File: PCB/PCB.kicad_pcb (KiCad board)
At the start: 2 copper layers, 3 parts, among them U3 PC817, U4 MAX31855KASA

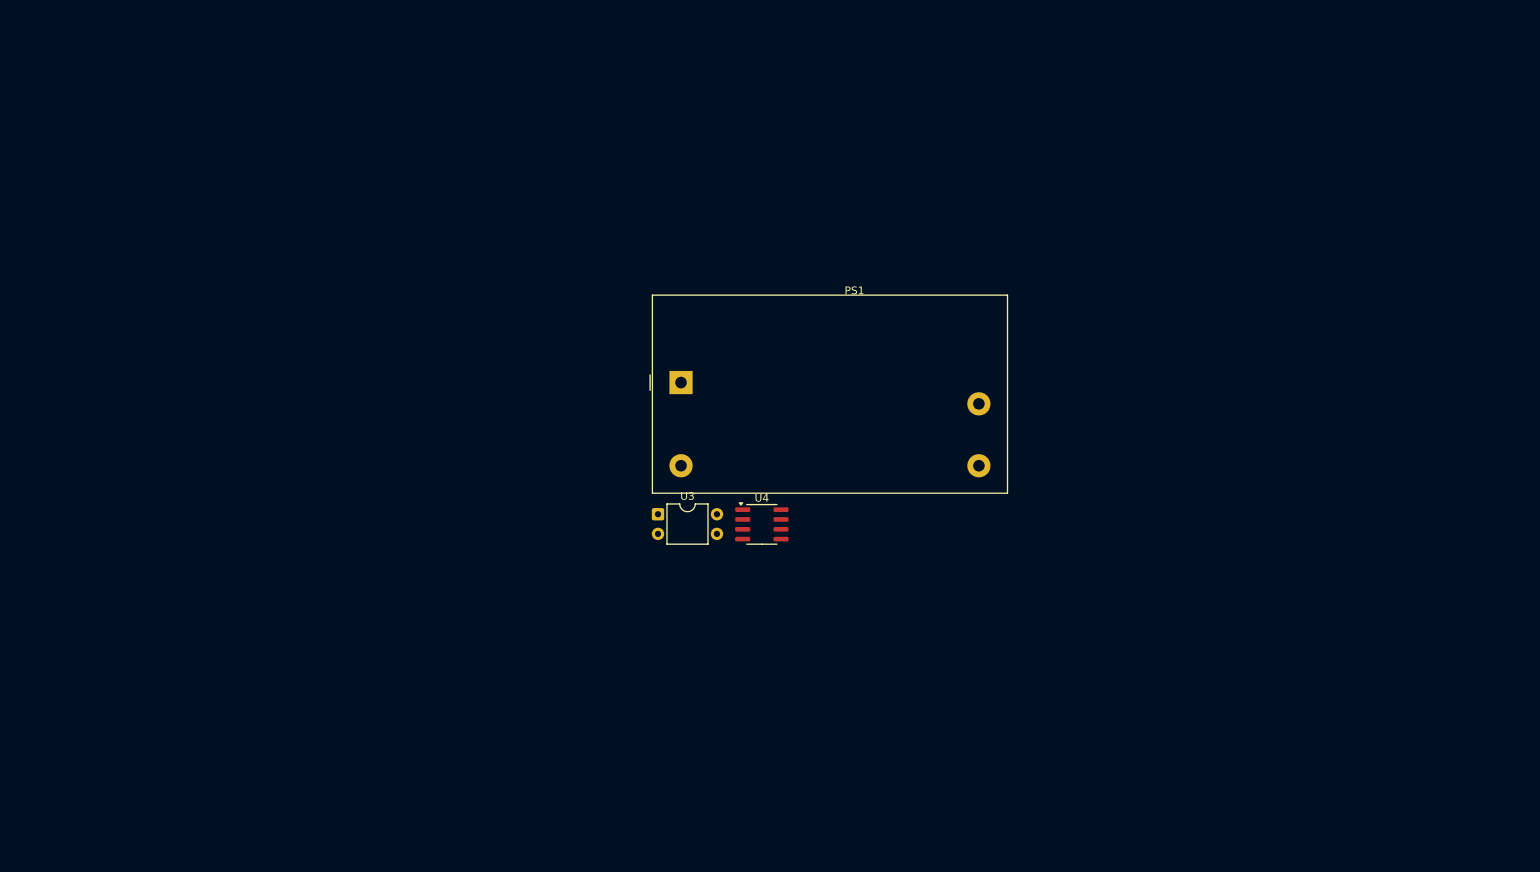
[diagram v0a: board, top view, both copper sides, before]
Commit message: add all the changes i've made, sorry for not gitting it bit by bit
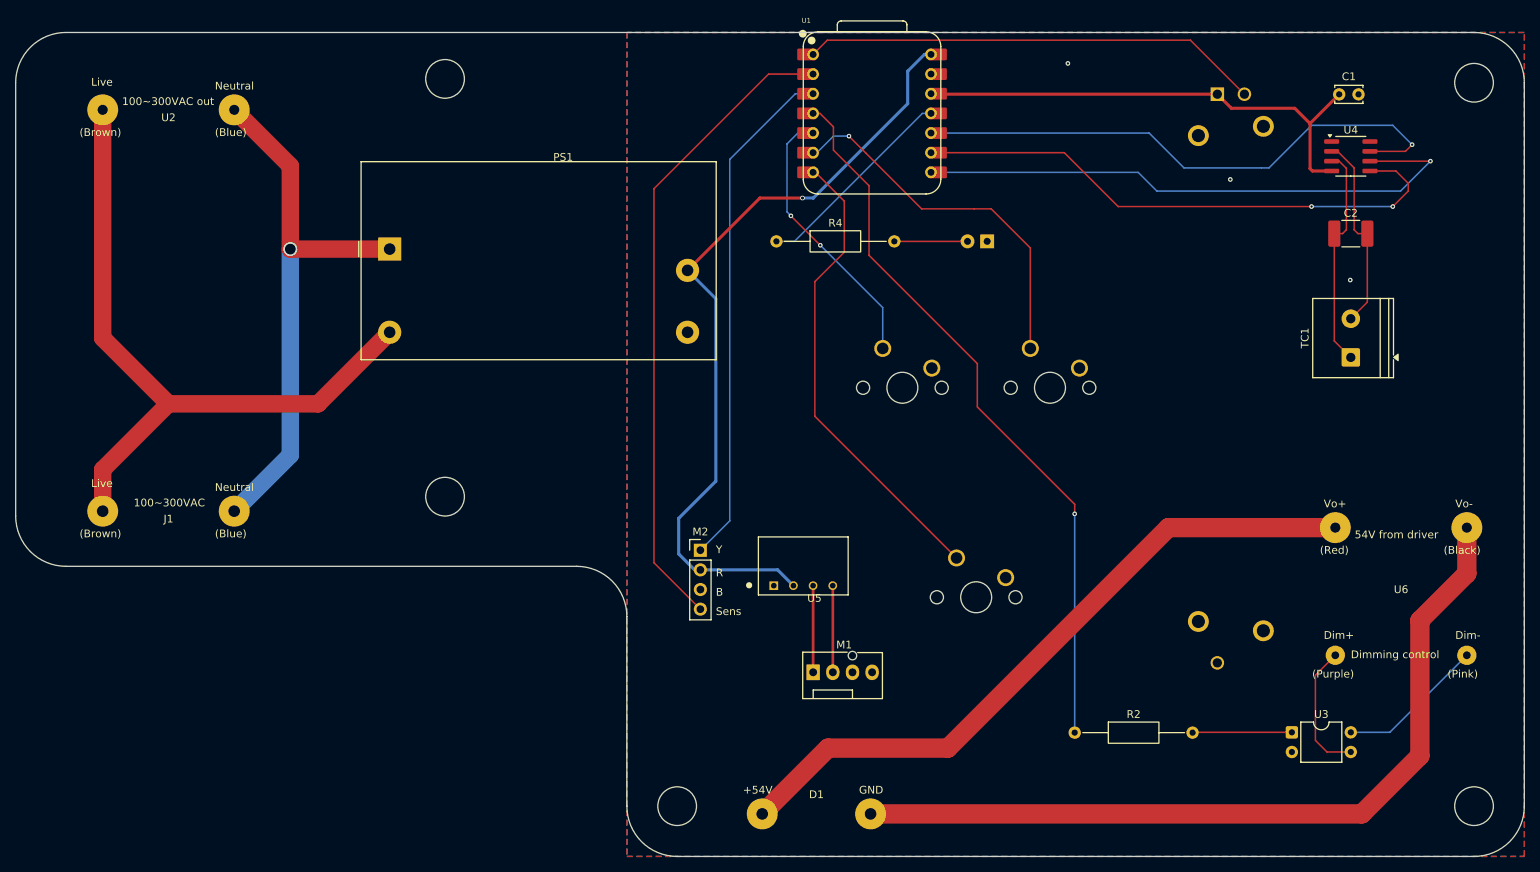
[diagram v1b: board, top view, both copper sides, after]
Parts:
- added C1: 0.1µF, Capacitor_THT:C_Disc_D3.4mm_W2.1mm_P2.50mm, F.Cu at (198.6, 40.0)
- added C2: 10nF, Capacitor_SMD:C_1812_4532Metric_Pad1.57x3.40mm_HandSolder, F.Cu at (200.1, 58.0)
- added D1: LED, custom footprints and stuff:Big Lumileds LED, F.Cu at (131.0, 137.5)
- added D2: LED red, LED_THT:LED_D5.0mm, B.Cu at (153.1, 59.0)
- added J1: IEC_C14_Receptacle, custom footprints and stuff:C14 Power input, F.Cu at (47.2, 97.9)
- added M1: Fan_4pin, Connector:FanPinHeader_1x04_P2.54mm_Vertical, F.Cu at (130.6, 114.7)
- added M2: Motor_Servo, Connector_PinHeader_2.54mm:PinHeader_1x04_P2.54mm_Vertical, F.Cu at (116.0, 98.9)
- added R2: 42Ω 0.12W, Resistor_THT:R_Axial_DIN0207_L6.3mm_D2.5mm_P15.24mm_Horizontal, F.Cu at (164.4, 122.5)
- added R4: 40-60Ω, Resistor_THT:R_Axial_DIN0207_L6.3mm_D2.5mm_P15.24mm_Horizontal, F.Cu at (125.8, 59.0)
- added RV1: Pot, Potentiometer_THT:Potentiometer_Bourns_PTA6043_Single_Slide, B.Cu at (182.8, 40.0)
- added SW2: SW_Push SET, Button_Switch_Keyboard:SW_Cherry_MX_1.00u_PCB, B.Cu at (149.1, 99.9)
- added SW3: SW_Push Pos1, Button_Switch_Keyboard:SW_Cherry_MX_1.00u_PCB, B.Cu at (158.7, 72.8)
- added SW4: SW_Push Pos2, Button_Switch_Keyboard:SW_Cherry_MX_1.00u_PCB, B.Cu at (139.6, 72.8)
- added TC1: Thermocouple_Block, TerminalBlock_Philmore:TerminalBlock_Philmore_TB132_1x02_P5.00mm_Horizontal, F.Cu at (200.1, 74.0)
- added U1: XIAO-RP2040-DIP, Seeed Studio XIAO Series Library:XIAO-RP2040-DIP, F.Cu at (138.2, 42.5)
- added U2: Meanwell ELG-150-54B AC Side, custom footprints and stuff:Meanwell ELG-150-54B AC side, F.Cu at (47.2, 46.0)
- added U5: SMU02L-12, SMU02L_12:SIP750W50P254L1160H1014Q4, F.Cu at (129.3, 101.0)
- added U6: Meanwell ELG-150-54B Other side, custom footprints and stuff:Meanwell ELG-150-54B Other Side, F.Cu at (206.6, 100.0)
- moved U4 89.8 mm to (200.1, 48.0)
- moved U3 86.6 mm to (192.4, 122.5)
- moved PS1 41.4 mm to (75.8, 60.0)
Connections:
- U4 pad 2: GND -> Net-(TC1--)
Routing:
- net Net-(D1-K): track 0.00 -> 106.1 mm
- net +5V: track 0.00 -> 102.2 mm, vias 0 -> 1
- net Net-(U1-GPIO29/ADC3/A3): track 0.00 -> 94.6 mm, vias 0 -> 1
- net Net-(J1-L): track 0.00 -> 91.3 mm
- net Net-(D1-A): track 0.00 -> 89.4 mm
- net Net-(M2-Sense): track 0.00 -> 82.7 mm
- net Net-(U1-GPIO1/RX): track 0.00 -> 75.0 mm, vias 0 -> 1
- net Net-(U1-GPIO4/MISO): track 0.00 -> 73.2 mm, vias 0 -> 1
- net Net-(U1-GPIO2/SCK): track 0.00 -> 71.2 mm, vias 0 -> 2
- net Net-(J1-N): track 0.00 -> 70.7 mm, vias 0 -> 1
- net Net-(M2-PWM): track 0.00 -> 66.4 mm
- net +3V3: track 0.00 -> 63.8 mm
- net Net-(U1-GPIO0/TX): track 0.00 -> 60.8 mm
- net Net-(U1-GPIO26/ADC0/A0): track 0.00 -> 59.4 mm
- net Net-(U1-GPIO7/SCL): track 0.00 -> 47.9 mm, vias 0 -> 1
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- added copper zone on B.Cu, net GND
- added copper zone on F.Cu, net GND
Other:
- board outline added: 195 x 106.5 mm

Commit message: uhh did stuff by the looks of it
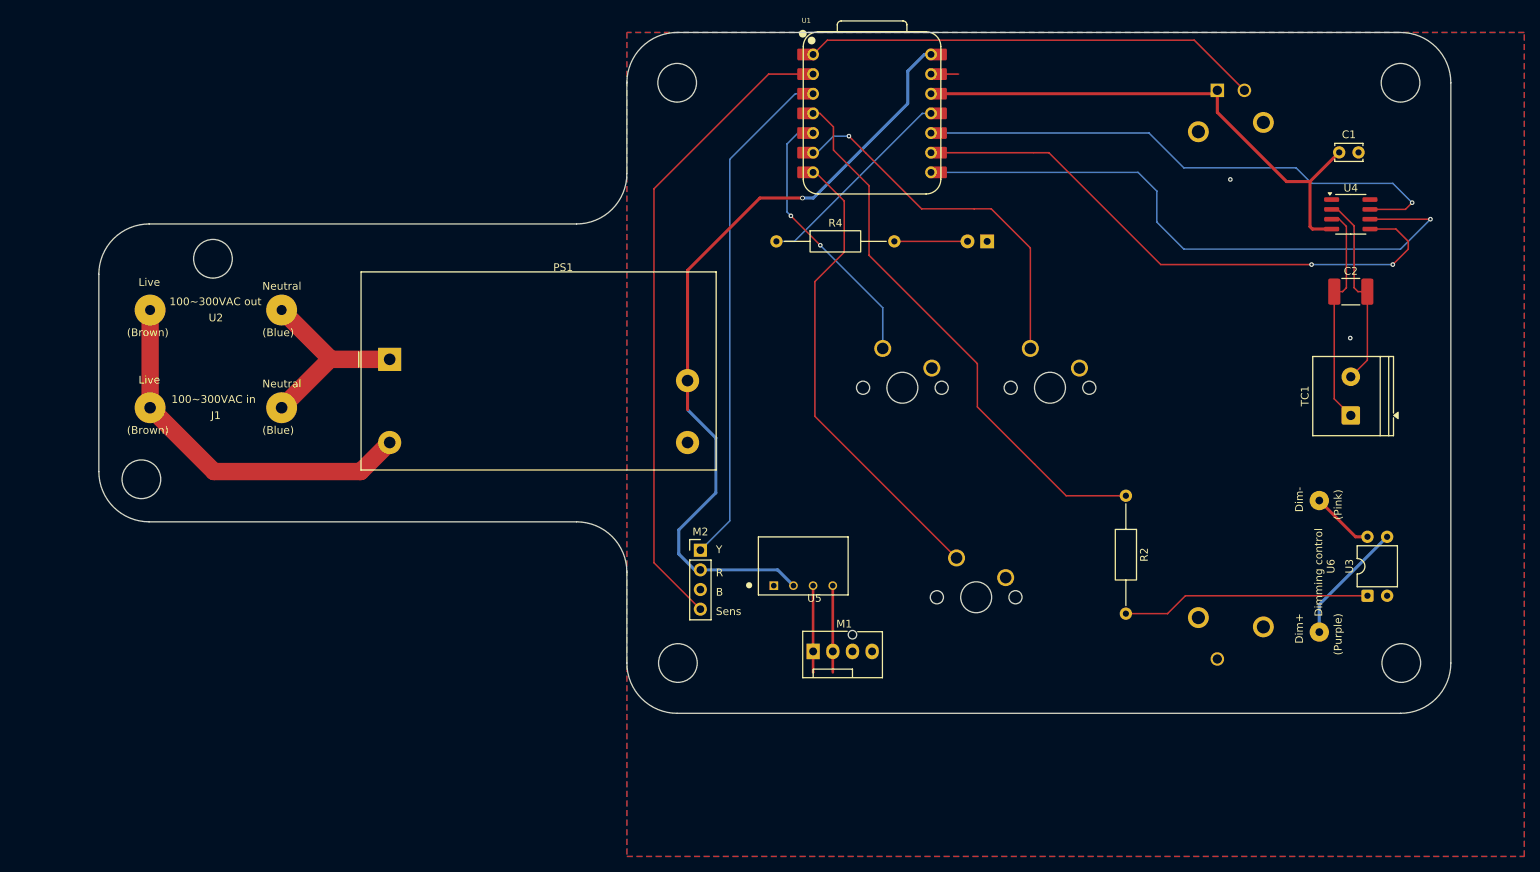
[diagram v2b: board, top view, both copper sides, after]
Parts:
- removed D1: LED, custom footprints and stuff:Big Lumileds LED
- moved R2 31.3 mm to (171.0, 91.9), turned to -90 degrees
- moved U2 26.6 mm to (53.4, 71.9)
- moved U6 23.1 mm to (183.5, 101.0), turned to 90 degrees
- moved U3 20.2 mm to (202.2, 104.8), turned to 90 degrees
- moved J1 14.7 mm to (53.4, 84.5)
- moved PS1 14.2 mm to (75.8, 74.2)
- moved C1 7.50 mm to (198.6, 47.5)
- moved C2 7.50 mm to (200.1, 65.5)
- moved TC1 7.50 mm to (200.1, 81.5)
- moved U4 7.50 mm to (200.1, 55.5)
- moved M1 2.70 mm to (130.6, 112.0)
- moved RV1 0.50 mm to (182.8, 39.5)
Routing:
- net Net-(D1-K): track 106.1 -> 0.00 mm
- net Net-(D1-A): track 89.4 -> 0.00 mm
- net Net-(J1-N): track 70.7 -> 25.6 mm, vias 1 -> 0
- net Net-(J1-L): track 91.3 -> 48.4 mm
- net Net-(U1-GPIO29/ADC3/A3): track 94.6 -> 71.2 mm, vias 1 -> 0
- net Net-(R2-Pad2): track 12.8 -> 32.2 mm
- net Net-(U6-Dim-): track 19.1 -> 8.17 mm
- net Net-(U1-GPIO1/RX): track 75.0 -> 80.4 mm
- net +3V3: track 63.8 -> 69.0 mm
- net Net-(U1-GPIO2/SCK): track 71.2 -> 74.3 mm
- net GND: track 0.00 -> 2.73 mm, vias 3 -> 2
- net Net-(U1-GPIO4/MISO): track 73.2 -> 71.7 mm
- net Net-(U6-Dim+): track 17.3 -> 15.9 mm
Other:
- board size 195 x 106.5 mm -> 174.8 x 88 mm
